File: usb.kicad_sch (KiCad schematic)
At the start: 8 parts, among them J4 USB3_DOUBLE, J5 HDMI_FRONT, U4 USB5744T/2GX01, U7 DISPLAYPORT_DOUBLE, U8 DP_REAR

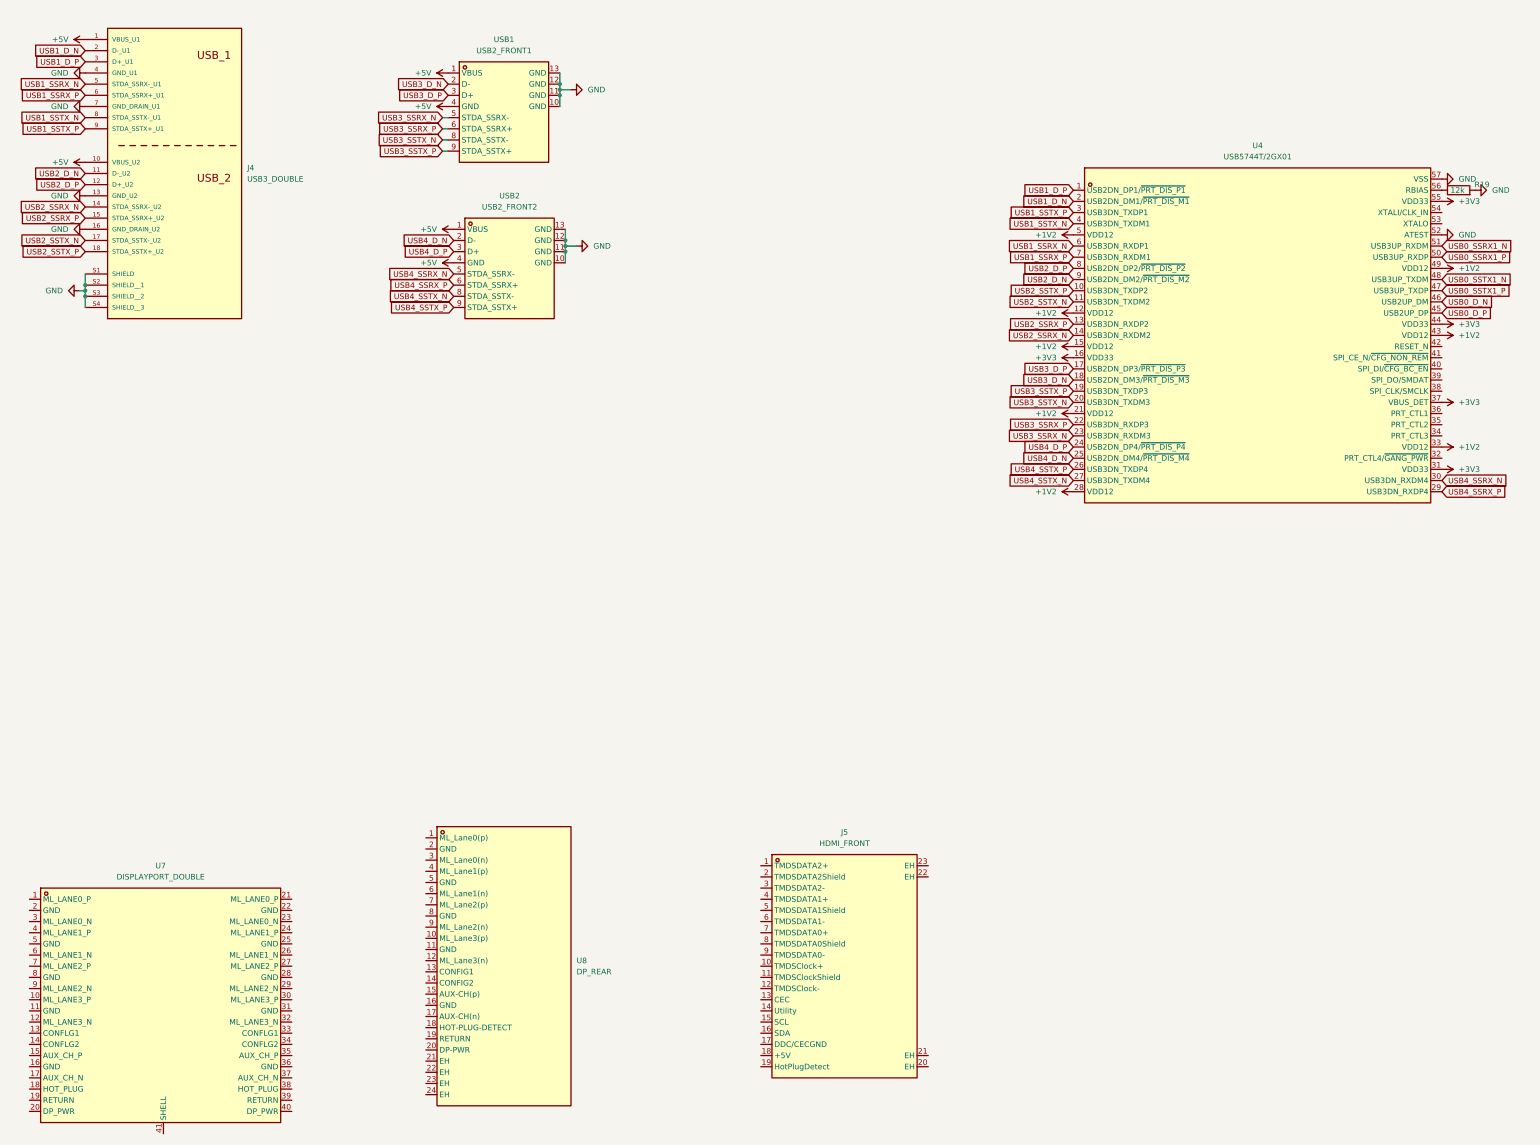
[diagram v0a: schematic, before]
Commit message: update readme.md
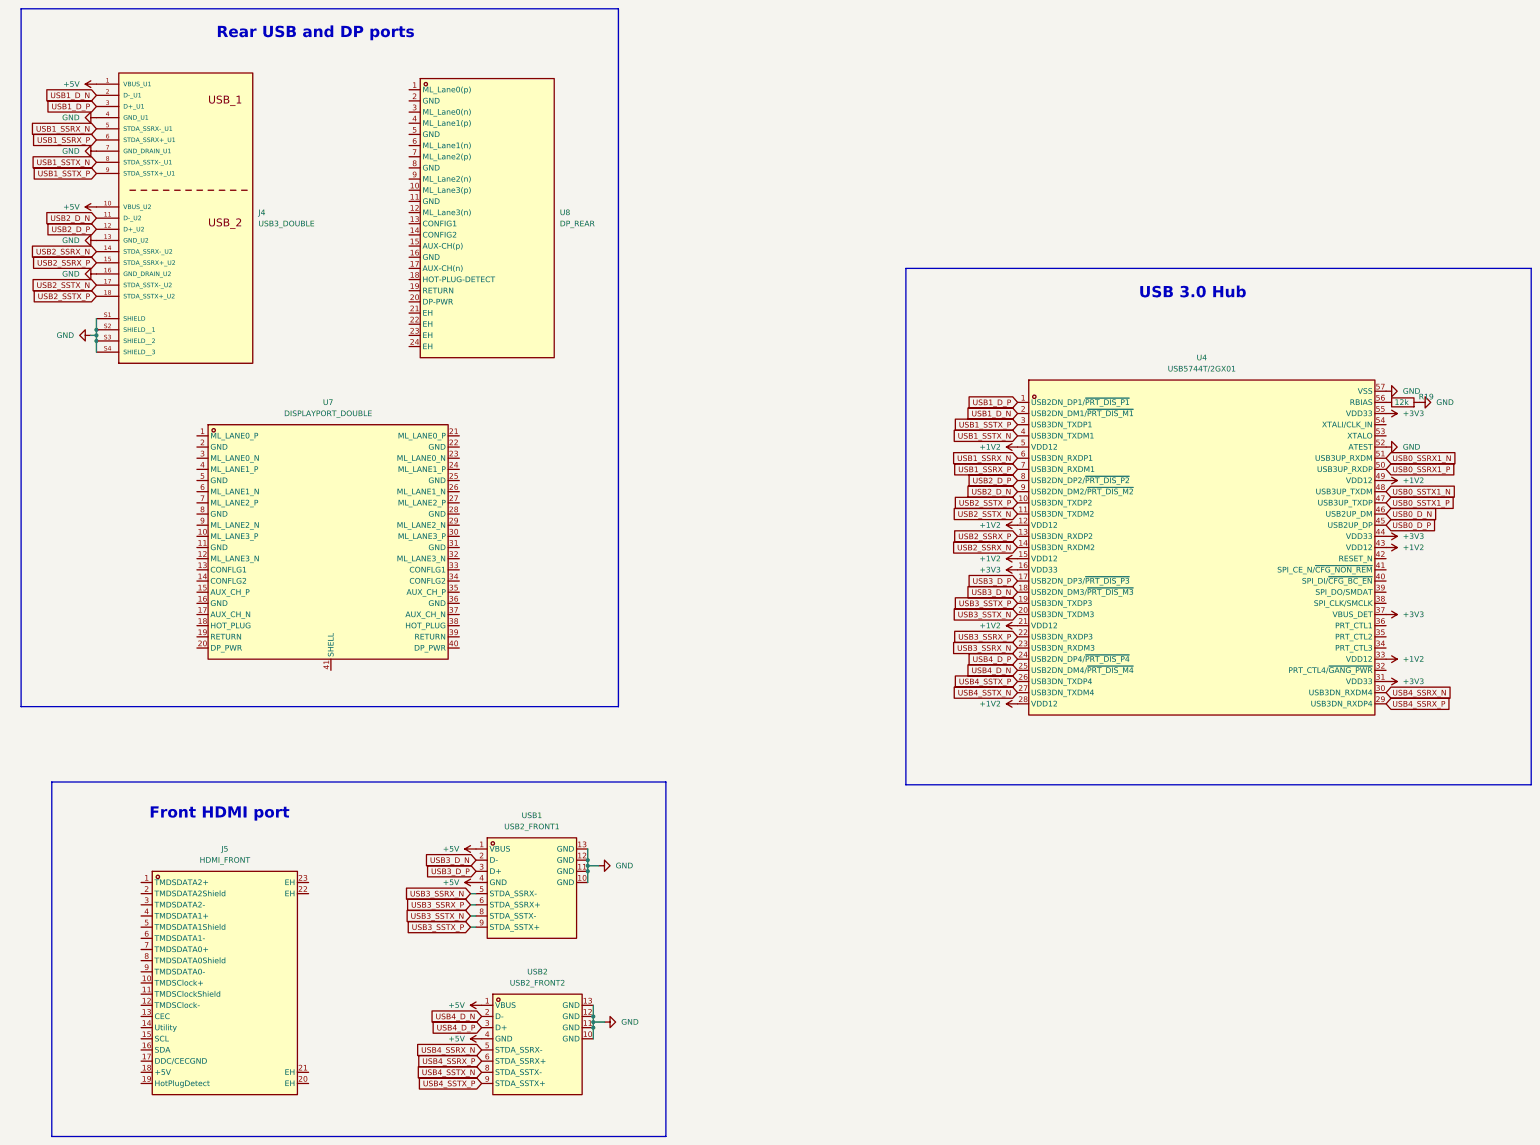
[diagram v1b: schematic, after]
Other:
- note added: "Front HDMI port"
- note added: "Rear USB and DP ports"
- note added: "USB 3.0 Hub"
- company: (none) -> mothenjoyer69
- title: (none) -> ThunderMXM
- moved on the sheet: J4, J5, R19, U4, U7, U8, USB1, USB2
